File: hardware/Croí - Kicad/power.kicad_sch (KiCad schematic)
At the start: 22 parts, among them U6 MPM3650CGQW-P

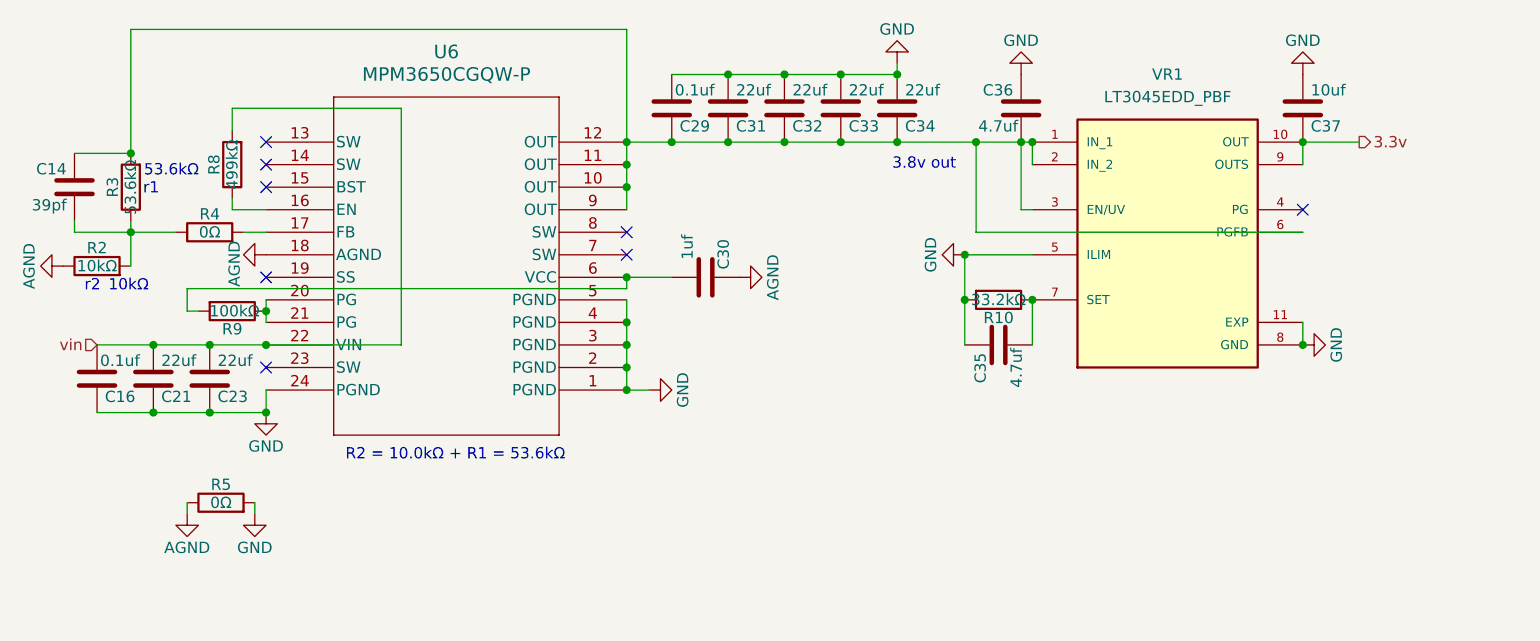
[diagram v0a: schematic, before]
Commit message: running
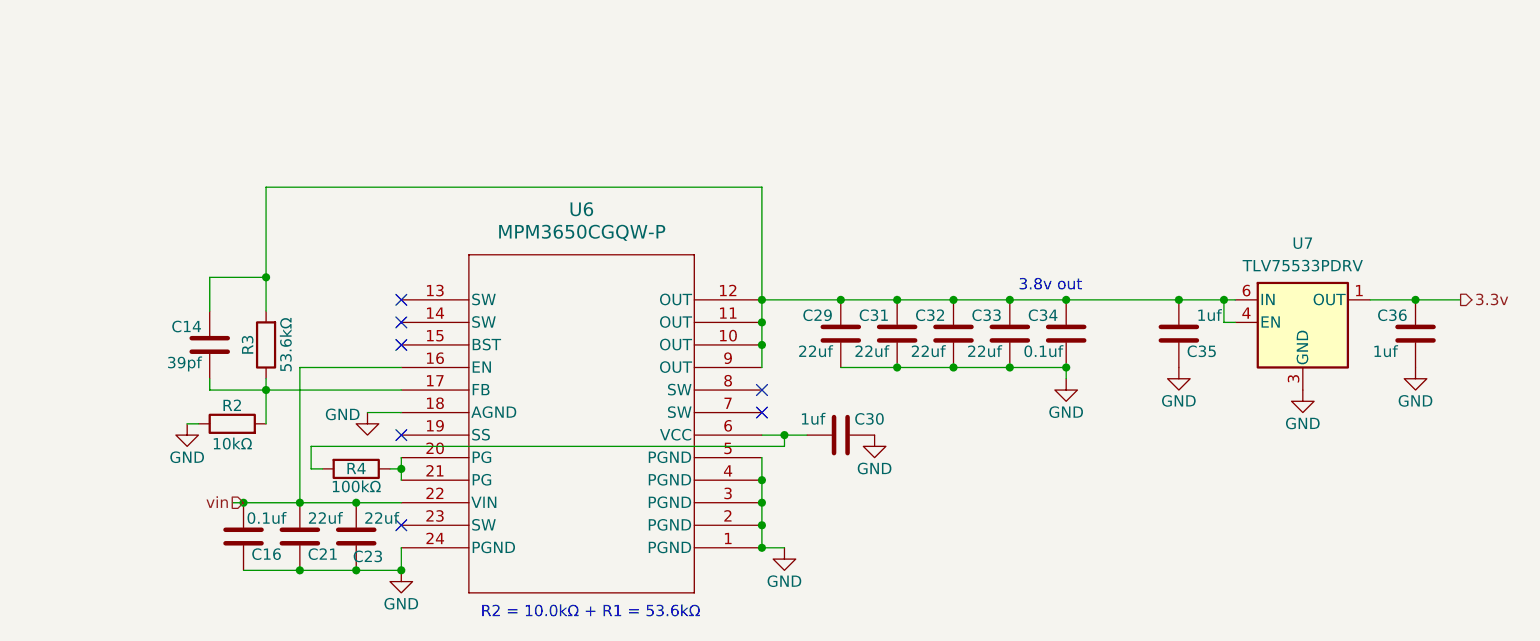
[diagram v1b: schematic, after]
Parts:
- removed C35: 4.7uf, Capacitor_SMD:C_0402_1005Metric, symbol Device:C
- removed R10: 33.2kΩ, Resistor_SMD:R_0402_1005Metric, symbol Device:R
- removed R4, R5: 0Ω, Resistor_SMD:R_0402_1005Metric, symbol Device:R
- removed R8: 499kΩ, Resistor_SMD:R_0402_1005Metric, symbol Device:R
- removed VR1: LT3045EDD_PBF, SON50P300X300X80-11N, symbol LT3045EDD_PBF:LT3045EDD_PBF
- added U7: TLV75533PDRV, Package_SON:WSON-6-1EP_2x2mm_P0.65mm_EP1x1.6mm, symbol Regulator_Linear:TLV75533PDRV
- C35: renamed from C36; value 4.7uf -> 1uf
- C36: renamed from C37; value 10uf -> 1uf
- renumbered C34 to C29, C33 to C31, C31 to C33, C29 to C34, R9 to R4
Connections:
- net AGND is gone; now on net GND: C30.1, R2.1, U6.18 (AGND)
- net 3.3v: now also U7.1 (OUT)
- net GND: now also U7.3 (GND), U7.7 (GND)
- net vin: now also U6.16 (EN)
- net at C14.2, R2.2, R3.1: now also U6.17 (FB)
- net at C14.1, C29.1, C31.1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: now also U7.4 (EN), U7.6 (IN)
- no-connect marks 8 -> 7
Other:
- note removed: "10kΩ"
- note removed: "53.6kΩ"
- note removed: "r1"
- note removed: "r2"
- moved on the sheet: C14, C16, C21, C23, C29, C30, C31, C32, C33, C34, C35, C36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

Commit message: progress, not flashing yet
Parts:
- C21, C23, C29, C31, C32, C33: footprint Capacitor_SMD:C_0402_1005Metric -> Capacitor_SMD:C_0603_1608Metric
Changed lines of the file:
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@@
 			)
 		)
-		(property "Footprint" "Capacitor_SMD:C_0402_1005Metric"
+		(property "Footprint" "Capacitor_SMD:C_0603_1608Metric"
 			(at 67.6148 104.14 0)
 			(effects
@@
 			)
 		)
+		(property "SNAPEDA_PN" ""
+			(at 68.58 107.95 0)
+			(effects
+				(font
+					(size 1.27 1.27)
+				)
+				(hide yes)
+			)
+		)
 		(pin "1"
 		)
@@
 			)
 		)
+		(property "SNAPEDA_PN" ""
+			(at 62.23 107.95 0)
+			(effects
+				(font
+					(size 1.27 1.27)
+				)
+				(hide yes)
+			)
+		)
 		(pin "1"
 		)
@@
 			)
 		)
+		(property "SNAPEDA_PN" ""
+			(at 154.94 85.09 0)
+			(effects
+				(font
+					(size 1.27 1.27)
+				)
+				(hide yes)
+			)
+		)
 		(pin "1"
 		)
@@
 			)
 		)
-		(property "Footprint" "Capacitor_SMD:C_0402_1005Metric"
+		(property "Footprint" "Capacitor_SMD:C_0603_1608Metric"
 			(at 130.5052 88.9 0)
 			(effects
@@
 			)
 		)
+		(property "SNAPEDA_PN" ""
+			(at 129.54 85.09 0)
+			(effects
+				(font
+					(size 1.27 1.27)
+				)
+				(hide yes)
+			)
+		)
 		(pin "1"
 		)
@@
 			)
 		)
+		(property "SNAPEDA_PN" ""
+			(at 194.31 85.09 0)
+			(effects
+				(font
+					(size 1.27 1.27)
+				)
+				(hide yes)
+			)
+		)
 		(pin "1"
 		)
@@
 			)
 		)
+		(property "SNAPEDA_PN" ""
+			(at 74.93 100.33 90)
+			(effects
+				(font
+					(size 1.27 1.27)
+				)
+				(hide yes)
+			)
+		)
 		(pin "2"
 		)
@@
 			)
 		)
+		(property "SNAPEDA_PN" ""
+			(at 167.64 85.09 0)
+			(effects
+				(font
+					(size 1.27 1.27)
+				)
+				(hide yes)
+			)
+		)
 		(pin "1"
 		)
@@
 			)
 		)
-		(property "Footprint" "Capacitor_SMD:C_0402_1005Metric"
+		(property "Footprint" "Capacitor_SMD:C_0603_1608Metric"
 			(at 143.2052 88.9 0)
 			(effects
@@
 			)
 		)
+		(property "SNAPEDA_PN" ""
+			(at 142.24 85.09 0)
+			(effects
+				(font
+					(size 1.27 1.27)
+				)
+				(hide yes)
+			)
+		)
 		(pin "1"
 		)
@@
 			)
 		)
-		(property "Footprint" "Capacitor_SMD:C_0402_1005Metric"
+		(property "Footprint" "Capacitor_SMD:C_0603_1608Metric"
 			(at 149.5552 88.9 0)
 			(effects
@@
 			)
 		)
+		(property "SNAPEDA_PN" ""
+			(at 148.59 85.09 0)
+			(effects
+				(font
+					(size 1.27 1.27)
+				)
+				(hide yes)
+			)
+		)
 		(pin "1"
 		)
@@
 			)
 		)
+		(property "SNAPEDA_PN" ""
+			(at 129.54 96.52 90)
+			(effects
+				(font
+					(size 1.27 1.27)
+				)
+				(hide yes)
+			)
+		)
 		(pin "1"
 		)
@@
 		)
 		(property "Description" "Unpolarized capacitor"
+			(at 58.42 86.36 0)
+			(effects
+				(font
+					(size 1.27 1.27)
+				)
+				(hide yes)
+			)
+		)
+		(property "SNAPEDA_PN" ""
 			(at 58.42 86.36 0)
 			(effects
@@
 			)
 		)
+		(property "SNAPEDA_PN" ""
+			(at 120.65 109.22 0)
+			(effects
+				(font
+					(size 1.27 1.27)
+				)
+				(hide yes)
+			)
+		)
 		(pin "10"
 		)
@@
 		(property "Description" "Resistor"
 			(at 60.96 95.25 0)
+			(effects
+				(font
+					(size 1.27 1.27)
+				)
+				(hide yes)
+			)
+		)
+		(property "SNAPEDA_PN" ""
+			(at 60.96 95.25 90)
 			(effects
 				(font
@@
 			)
 		)
+		(property "SNAPEDA_PN" ""
+			(at 181.61 83.82 0)
+			(effects
+				(font
+					(size 1.27 1.27)
+				)
+				(hide yes)
+			)
+		)
 		(pin "1"
 		)
@@
 			)
 		)
-		(property "Footprint" "Capacitor_SMD:C_0402_1005Metric"
+		(property "Footprint" "Capacitor_SMD:C_0603_1608Metric"
 			(at 73.9648 104.14 0)
 			(effects
@@
 			)
 		)
+		(property "SNAPEDA_PN" ""
+			(at 74.93 107.95 0)
+			(effects
+				(font
+					(size 1.27 1.27)
+				)
+				(hide yes)
+			)
+		)
 		(pin "1"
 		)
@@
 			)
 		)
+		(property "SNAPEDA_PN" ""
+			(at 64.77 86.36 90)
+			(effects
+				(font
+					(size 1.27 1.27)
+				)
+				(hide yes)
+			)
+		)
 		(pin "2"
 		)
@@
 			)
 		)
-		(property "Footprint" "Capacitor_SMD:C_0402_1005Metric"
+		(property "Footprint" "Capacitor_SMD:C_0603_1608Metric"
 			(at 136.8552 88.9 0)
 			(effects
@@
 			(at 135.89 85.09 0)
 			(effects
+				(font
+					(size 1.27 1.27)
+				)
+				(hide yes)
+			)
+		)
+		(property "SNAPEDA_PN" ""
+			(at 135.89 85.09 0)
+			(effects
